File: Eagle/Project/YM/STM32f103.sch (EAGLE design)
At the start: 78 parts, among them IC1 YM3812, IC10 YM3812, IC11 YM3014B, IC12 LM358N, IC13 BA033CC0T, IC14 74ALS04N, IC15 6N136, IC2 YM3014B, IC3 LM358N, IC4 YM3812, IC5 YM3014B, IC6 LM358N, IC7 YM3812, IC8 YM3014B, IC9 LM358N, J2 DIN5, U1 STM32F10XRXT6, X1 CRYSTALS-NOGND-4-HSMX

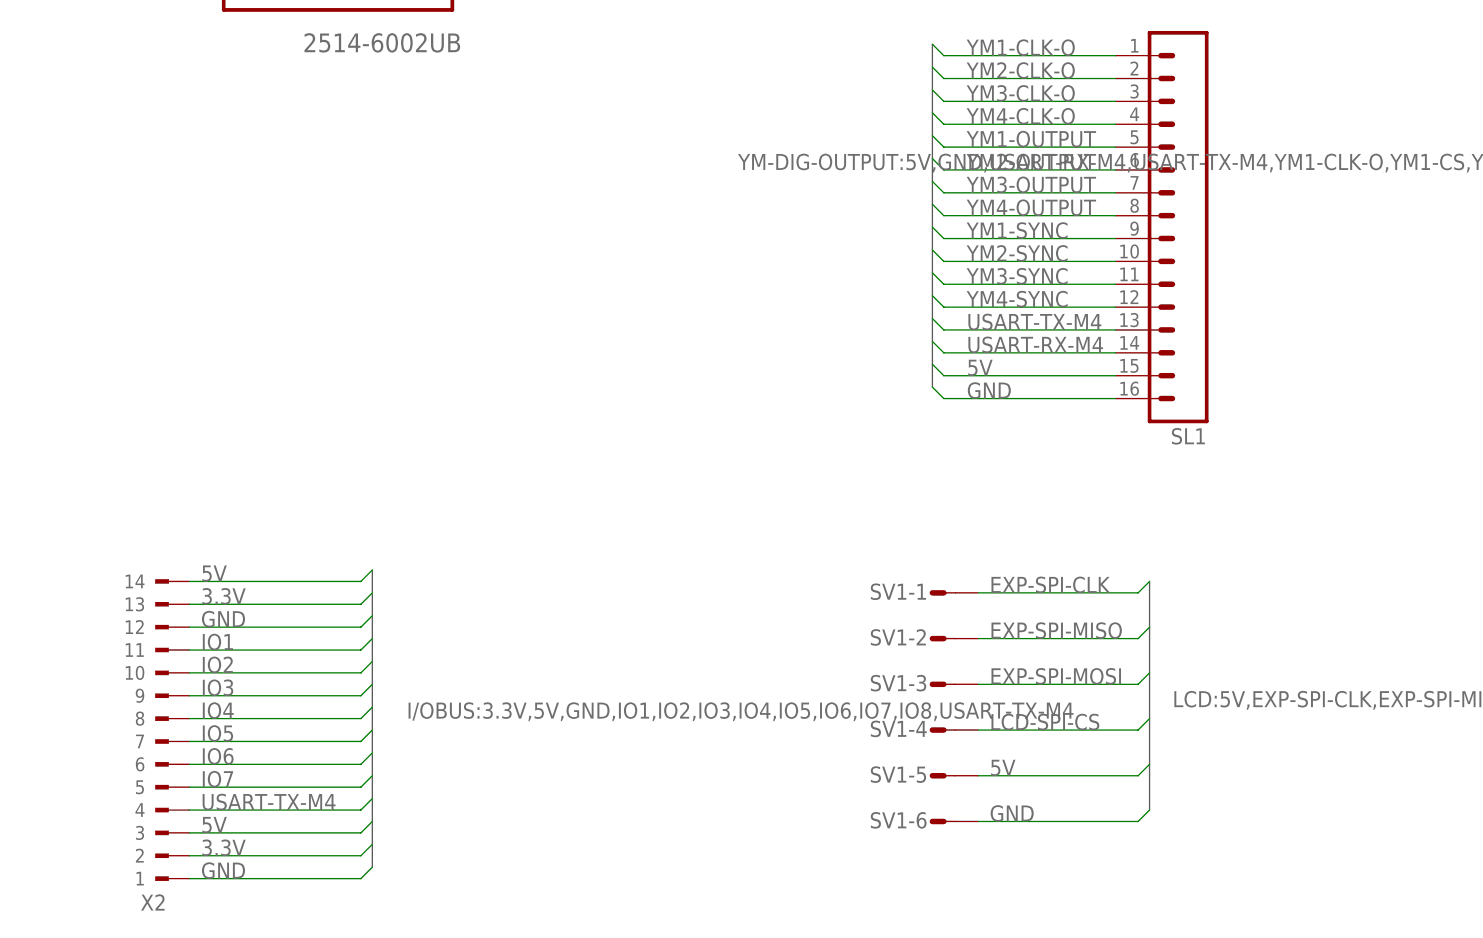
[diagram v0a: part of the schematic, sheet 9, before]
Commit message: v3.0 - PCB review aangepast
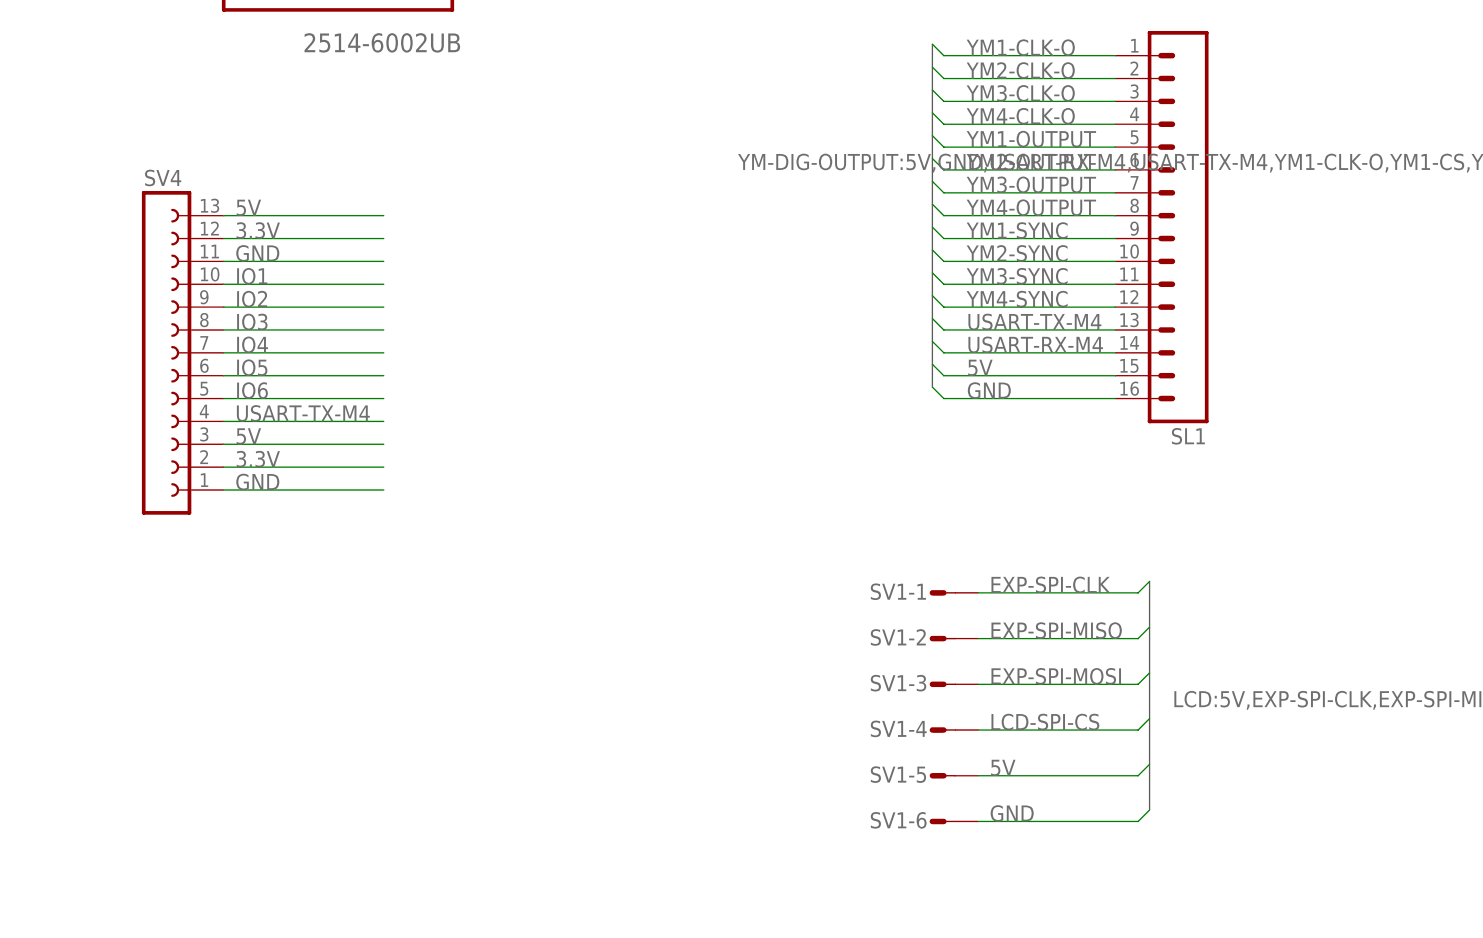
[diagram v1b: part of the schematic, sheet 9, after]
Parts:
- removed X2: (no value), con-weidmueller-sl35:180G-14
- added SV4: (no value), con-lsta:FE13-1
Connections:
- removed net IO7: X2.5
- net 3.3V: now also SV4.12, SV4.2; no longer X2.13, X2.2
- net 5V: now also SV4.13, SV4.3; no longer X2.14, X2.3
- net GND: now also SV4.1, SV4.11; no longer X2.1, X2.12
- net IO1: now also SV4.10; no longer X2.11
- net IO2: now also SV4.9; no longer X2.10
- net IO3: now also SV4.8; no longer X2.9
- net IO4: now also SV4.7; no longer X2.8
- net IO5: now also SV4.6; no longer X2.7
- net IO6: now also SV4.5; no longer X2.6
- net USART-TX-M4: now also SV4.4; no longer X2.4
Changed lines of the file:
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@@
 <part name="J9" library="con-amp" library_urn="urn:adsk.eagle:library:127" deviceset="MTA03-156" device="" package3d_urn="urn:adsk.eagle:package:8081563/1"/>
 <part name="J10" library="con-amp" library_urn="urn:adsk.eagle:library:127" deviceset="MTA03-156" device="" package3d_urn="urn:adsk.eagle:package:8081563/1"/>
-<part name="X2" library="con-weidmueller-sl35" library_urn="urn:adsk.eagle:library:199" deviceset="180G-14" device="" package3d_urn="urn:adsk.eagle:package:11378/1"/>
 <part name="J2" library="SparkFun-Connectors" library_urn="urn:adsk.eagle:library:513" deviceset="DIN5" device="" package3d_urn="urn:adsk.eagle:package:38294/1"/>
 <part name="D1" library="BAT20JFILM" deviceset="BAT20JFILM" device=""/>
@@
 <part name="SV2" library="con-lstb" library_urn="urn:adsk.eagle:library:162" deviceset="MA04-1" device="" package3d_urn="urn:adsk.eagle:package:8337/1"/>
 <part name="SV3" library="2514-6002UB" deviceset="2514-6002UB" device=""/>
+<part name="SV4" library="con-lsta" library_urn="urn:adsk.eagle:library:161" deviceset="FE13-1" device="" package3d_urn="urn:adsk.eagle:package:8213/1"/>
 </parts>
 <sheets>
@@
 <attribute name="VALUE" x="215.9" y="58.42" size="1.778" layer="96" rot="R270"/>
 </instance>
-<instance part="X2" gate="G$1" x="30.48" y="43.18" smashed="yes" rot="R180">
-<attribute name="NAME" x="30.48" y="26.162" size="1.778" layer="95" rot="R180"/>
-<attribute name="VALUE" x="30.48" y="64.516" size="1.778" layer="96" rot="R180"/>
-</instance>
 <instance part="SL2" gate="G$1" x="140.97" y="142.24" smashed="yes" rot="R180">
 <attribute name="VALUE" x="146.05" y="152.4" size="1.778" layer="96" rot="R180"/>
@@
 <attribute name="VALUE" x="45.6184" y="119.761" size="2.0828" layer="96" ratio="10" rot="SR0"/>
 </instance>
+<instance part="SV4" gate="G$1" x="29.21" y="86.36" smashed="yes">
+<attribute name="VALUE" x="27.94" y="66.04" size="1.778" layer="96"/>
+<attribute name="NAME" x="27.94" y="104.902" size="1.778" layer="95"/>
+</instance>
 </instances>
 <busses>
@@
 </segment>
 </bus>
-<bus name="I/OBUS:3.3V,5V,GND,IO1,IO2,IO3,IO4,IO5,IO6,IO7,IO8,USART-TX-M4">
-<segment>
-<wire x1="53.34" y1="62.23" x2="53.34" y2="29.21" width="0.762" layer="92"/>
-<label x="57.15" y="45.72" size="1.778" layer="95"/>
-</segment>
-</bus>
 <bus name="YM-DIG-OUTPUT:5V,GND,USART-RX-M4,USART-TX-M4,YM1-CLK-O,YM1-CS,YM1-OUTPUT,YM1-SYNC,YM2-CLK-O,YM2-OUTPUT,YM2-SYNC,YM3-CLK-O,YM3-OUTPUT,YM3-SYNC,YM4-CLK-O,YM4-OUTPUT,YM4-SYNC">
 <segment>
@@
 <net name="5V" class="0">
 <segment>
-<wire x1="33.02" y1="60.96" x2="52.07" y2="60.96" width="0.1524" layer="91"/>
-<wire x1="52.07" y1="60.96" x2="53.34" y2="62.23" width="0.1524" layer="91"/>
-<label x="34.29" y="60.96" size="1.778" layer="95"/>
-<pinref part="X2" gate="G$1" pin="14"/>
-</segment>
-<segment>
-<pinref part="X2" gate="G$1" pin="3"/>
-<wire x1="33.02" y1="33.02" x2="52.07" y2="33.02" width="0.1524" layer="91"/>
-<wire x1="52.07" y1="33.02" x2="53.34" y2="34.29" width="0.1524" layer="91"/>
-<label x="34.29" y="33.02" size="1.778" layer="95"/>
-</segment>
-<segment>
 <pinref part="SL1" gate="G$1" pin="15"/>
 <wire x1="135.89" y1="83.82" x2="116.84" y2="83.82" width="0.1524" layer="91"/>
@@
 <wire x1="31.75" y1="142.24" x2="13.97" y2="142.24" width="0.1524" layer="91"/>
 </segment>
+<segment>
+<pinref part="SV4" gate="G$1" pin="13"/>
+<wire x1="36.83" y1="101.6" x2="54.61" y2="101.6" width="0.1524" layer="91"/>
+<label x="38.1" y="101.6" size="1.778" layer="95"/>
+</segment>
+<segment>
+<pinref part="SV4" gate="G$1" pin="3"/>
+<wire x1="36.83" y1="76.2" x2="54.61" y2="76.2" width="0.1524" layer="91"/>
+<label x="38.1" y="76.2" size="1.778" layer="95"/>
+</segment>
 </net>
 <net name="3.3V" class="0">
@@
 </segment>
 <segment>
-<wire x1="33.02" y1="58.42" x2="52.07" y2="58.42" width="0.1524" layer="91"/>
-<wire x1="52.07" y1="58.42" x2="53.34" y2="59.69" width="0.1524" layer="91"/>
-<label x="34.29" y="58.42" size="1.778" layer="95"/>
-<pinref part="X2" gate="G$1" pin="13"/>
-</segment>
-<segment>
-<pinref part="X2" gate="G$1" pin="2"/>
-<wire x1="33.02" y1="30.48" x2="52.07" y2="30.48" width="0.1524" layer="91"/>
-<wire x1="52.07" y1="30.48" x2="53.34" y2="31.75" width="0.1524" layer="91"/>
-<label x="34.29" y="30.48" size="1.778" layer="95"/>
-</segment>
-<segment>
 <wire x1="218.44" y1="48.26" x2="198.12" y2="48.26" width="0.1524" layer="91"/>
 <wire x1="198.12" y1="48.26" x2="196.85" y2="49.53" width="0.1524" layer="91"/>
@@
 <wire x1="67.31" y1="142.24" x2="85.09" y2="142.24" width="0.1524" layer="91"/>
 </segment>
+<segment>
+<pinref part="SV4" gate="G$1" pin="12"/>
+<wire x1="36.83" y1="99.06" x2="54.61" y2="99.06" width="0.1524" layer="91"/>
+<label x="38.1" y="99.06" size="1.778" layer="95"/>
+</segment>
+<segment>
+<pinref part="SV4" gate="G$1" pin="2"/>
+<wire x1="36.83" y1="73.66" x2="54.61" y2="73.66" width="0.1524" layer="91"/>
+<label x="38.1" y="73.66" size="1.778" layer="95"/>
+</segment>
 </net>
 <net name="GND" class="0">
@@
 </segment>
 <segment>
-<wire x1="33.02" y1="55.88" x2="52.07" y2="55.88" width="0.1524" layer="91"/>
-<wire x1="52.07" y1="55.88" x2="53.34" y2="57.15" width="0.1524" layer="91"/>
-<label x="34.29" y="55.88" size="1.778" layer="95"/>
-<pinref part="X2" gate="G$1" pin="12"/>
-</segment>
-<segment>
-<pinref part="X2" gate="G$1" pin="1"/>
-<wire x1="33.02" y1="27.94" x2="52.07" y2="27.94" width="0.1524" layer="91"/>
-<wire x1="52.07" y1="27.94" x2="53.34" y2="29.21" width="0.1524" layer="91"/>
-<label x="34.29" y="27.94" size="1.778" layer="95"/>
-</segment>
-<segment>
 <wire x1="135.89" y1="134.62" x2="116.84" y2="134.62" width="0.1524" layer="91"/>
 <label x="119.38" y="134.62" size="1.778" layer="95"/>
@@
 <wire x1="67.31" y1="144.78" x2="85.09" y2="144.78" width="0.1524" layer="91"/>
 </segment>
+<segment>
+<pinref part="SV4" gate="G$1" pin="11"/>
+<wire x1="36.83" y1="96.52" x2="54.61" y2="96.52" width="0.1524" layer="91"/>
+<label x="38.1" y="96.52" size="1.778" layer="95"/>
+</segment>
+<segment>
+<pinref part="SV4" gate="G$1" pin="1"/>
+<wire x1="36.83" y1="71.12" x2="54.61" y2="71.12" width="0.1524" layer="91"/>
+<label x="38.1" y="71.12" size="1.778" layer="95"/>
+</segment>
 </net>
 <net name="ADC-VOL-TOT" class="0">
@@
 <net name="IO1" class="0">
 <segment>
-<wire x1="33.02" y1="53.34" x2="52.07" y2="53.34" width="0.1524" layer="91"/>
-<wire x1="52.07" y1="53.34" x2="53.34" y2="54.61" width="0.1524" layer="91"/>
-<label x="34.29" y="53.34" size="1.778" layer="95"/>
-<pinref part="X2" gate="G$1" pin="11"/>
+<pinref part="SV4" gate="G$1" pin="10"/>
+<wire x1="36.83" y1="93.98" x2="54.61" y2="93.98" width="0.1524" layer="91"/>
+<label x="38.1" y="93.98" size="1.778" layer="95"/>
 </segment>
 </net>
 <net name="IO2" class="0">
 <segment>
-<wire x1="33.02" y1="50.8" x2="52.07" y2="50.8" width="0.1524" layer="91"/>
-<wire x1="52.07" y1="50.8" x2="53.34" y2="52.07" width="0.1524" layer="91"/>
-<label x="34.29" y="50.8" size="1.778" layer="95"/>
-<pinref part="X2" gate="G$1" pin="10"/>
+<pinref part="SV4" gate="G$1" pin="9"/>
+<wire x1="36.83" y1="91.44" x2="54.61" y2="91.44" width="0.1524" layer="91"/>
+<label x="38.1" y="91.44" size="1.778" layer="95"/>
 </segment>
 </net>
 <net name="IO3" class="0">
 <segment>
-<wire x1="33.02" y1="48.26" x2="52.07" y2="48.26" width="0.1524" layer="91"/>
-<wire x1="52.07" y1="48.26" x2="53.34" y2="49.53" width="0.1524" layer="91"/>
-<label x="34.29" y="48.26" size="1.778" layer="95"/>
-<pinref part="X2" gate="G$1" pin="9"/>
+<pinref part="SV4" gate="G$1" pin="8"/>
+<wire x1="36.83" y1="88.9" x2="54.61" y2="88.9" width="0.1524" layer="91"/>
+<label x="38.1" y="88.9" size="1.778" layer="95"/>
 </segment>
 </net>
 <net name="IO4" class="0">
 <segment>
-<wire x1="33.02" y1="45.72" x2="52.07" y2="45.72" width="0.1524" layer="91"/>
-<wire x1="52.07" y1="45.72" x2="53.34" y2="46.99" width="0.1524" layer="91"/>
-<label x="34.29" y="45.72" size="1.778" layer="95"/>
-<pinref part="X2" gate="G$1" pin="8"/>
+<pinref part="SV4" gate="G$1" pin="7"/>
+<wire x1="36.83" y1="86.36" x2="54.61" y2="86.36" width="0.1524" layer="91"/>
+<label x="38.1" y="86.36" size="1.778" layer="95"/>
 </segment>
 </net>
 <net name="IO5" class="0">
 <segment>
-<wire x1="33.02" y1="43.18" x2="52.07" y2="43.18" width="0.1524" layer="91"/>
-<wire x1="52.07" y1="43.18" x2="53.34" y2="44.45" width="0.1524" layer="91"/>
-<pinref part="X2" gate="G$1" pin="7"/>
-<label x="34.29" y="43.18" size="1.778" layer="95"/>
+<pinref part="SV4" gate="G$1" pin="6"/>
+<wire x1="36.83" y1="83.82" x2="54.61" y2="83.82" width="0.1524" layer="91"/>
+<label x="38.1" y="83.82" size="1.778" layer="95"/>
 </segment>
 </net>
 <net name="IO6" class="0">
 <segment>
-<wire x1="33.02" y1="40.64" x2="52.07" y2="40.64" width="0.1524" layer="91"/>
-<wire x1="52.07" y1="40.64" x2="53.34" y2="41.91" width="0.1524" layer="91"/>
-<pinref part="X2" gate="G$1" pin="6"/>
-<label x="34.29" y="40.64" size="1.778" layer="95"/>
-</segment>
-</net>
-<net name="IO7" class="0">
-<segment>
-<wire x1="33.02" y1="38.1" x2="52.07" y2="38.1" width="0.1524" layer="91"/>
-<wire x1="52.07" y1="38.1" x2="53.34" y2="39.37" width="0.1524" layer="91"/>
-<pinref part="X2" gate="G$1" pin="5"/>
-<label x="34.29" y="38.1" size="1.778" layer="95"/>
+<pinref part="SV4" gate="G$1" pin="5"/>
+<wire x1="36.83" y1="81.28" x2="54.61" y2="81.28" width="0.1524" layer="91"/>
+<label x="38.1" y="81.28" size="1.778" layer="95"/>
 </segment>
 </net>
@@
 </segment>
 <segment>
-<pinref part="X2" gate="G$1" pin="4"/>
-<wire x1="33.02" y1="35.56" x2="52.07" y2="35.56" width="0.1524" layer="91"/>
-<wire x1="52.07" y1="35.56" x2="53.34" y2="36.83" width="0.1524" layer="91"/>
-<label x="34.29" y="35.56" size="1.778" layer="95"/>
+<pinref part="SV4" gate="G$1" pin="4"/>
+<wire x1="36.83" y1="78.74" x2="54.61" y2="78.74" width="0.1524" layer="91"/>
+<label x="38.1" y="78.74" size="1.778" layer="95"/>
 </segment>
 </net>
